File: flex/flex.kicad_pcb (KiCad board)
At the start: 2 copper layers, 68.2 x 125 mm, 11 parts, among them SW1 SW_Push, SW2 SW_Push, SW3 SW_Push

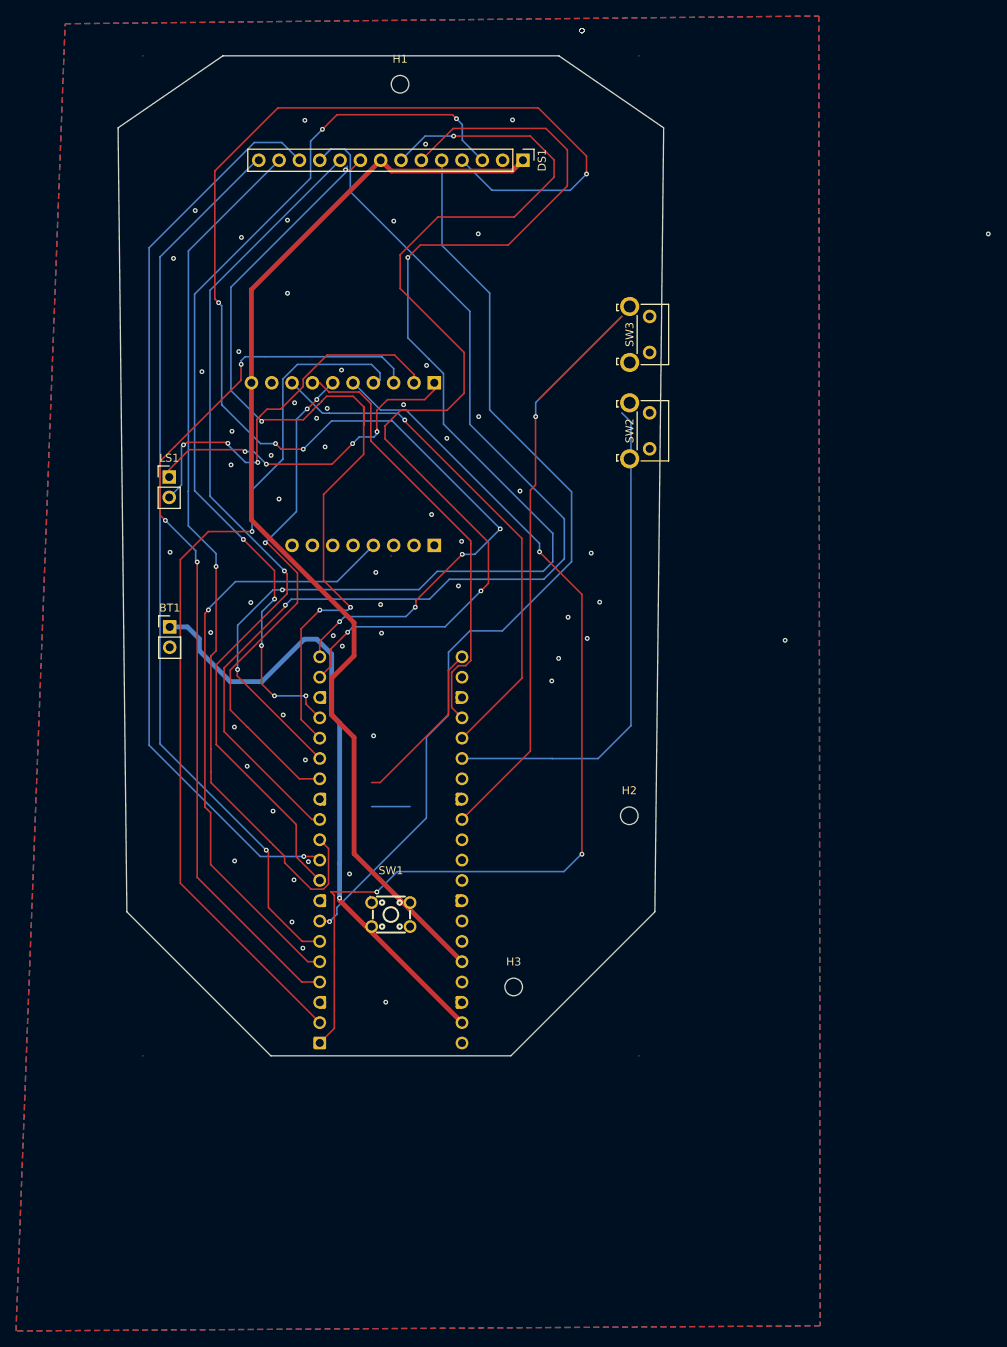
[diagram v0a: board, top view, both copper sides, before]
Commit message: started on firmware
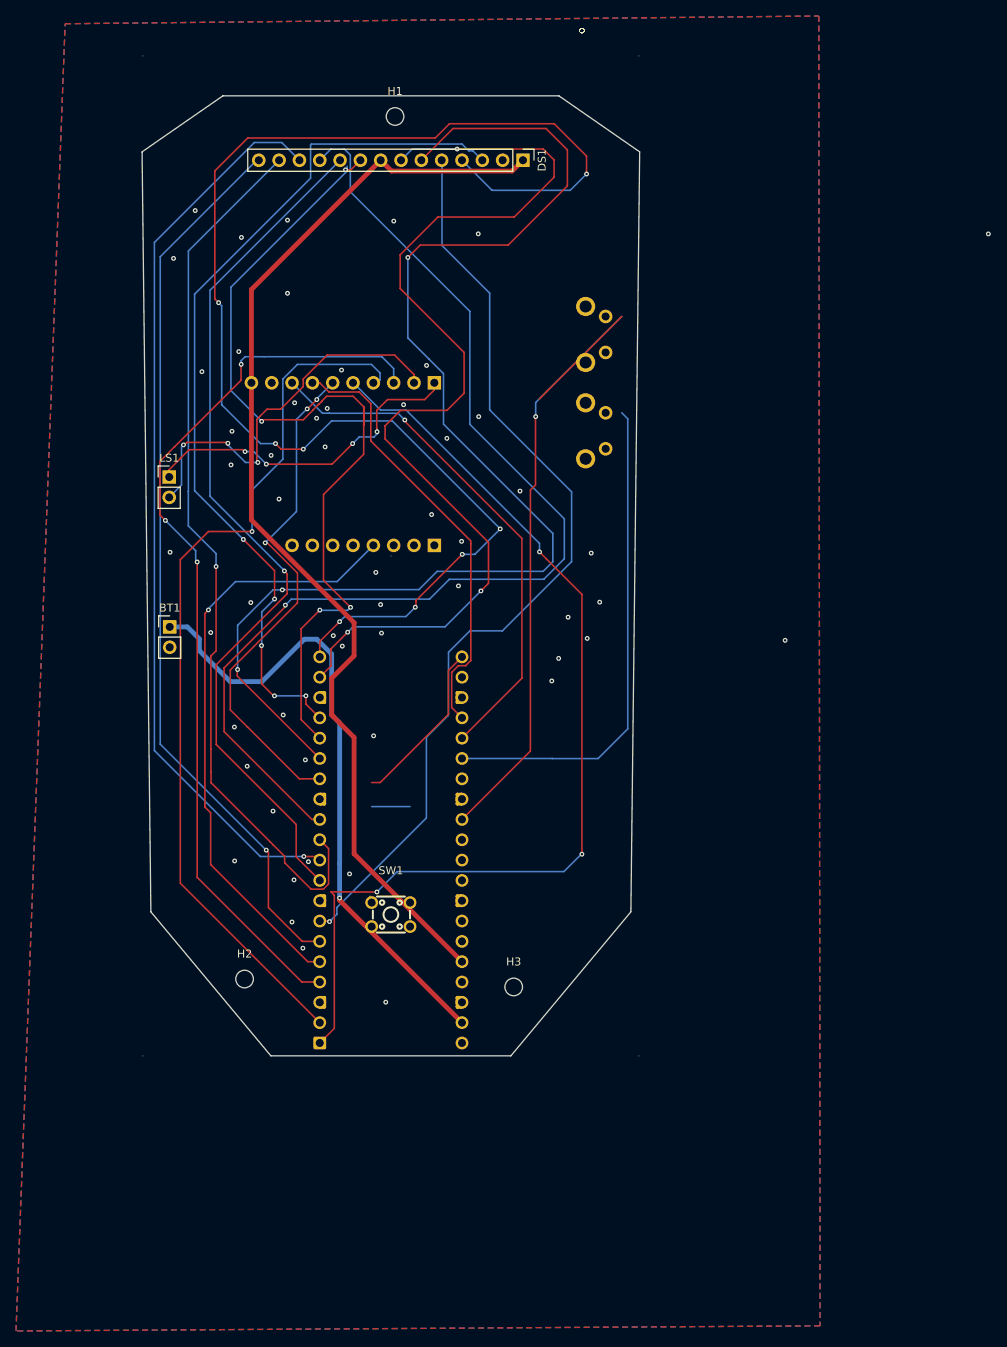
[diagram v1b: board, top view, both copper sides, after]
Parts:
- SW2, SW3: moved to B.Cu
- moved H2 52.2 mm to (84.8, 143.9)
- moved SW3 17.4 mm to (130.0, 77.7), turned to 90 degrees
- moved SW2 9.34 mm to (130.0, 65.6), turned to 90 degrees
- moved H1 4.08 mm to (103.6, 36.1)
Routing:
- net /DISP_CS: track 114.8 -> 110.3 mm, vias 7 -> 5
- net /DISP_RESET: track 177.1 -> 175.5 mm
- net /DISP_SCK: track 131.5 -> 130.1 mm
- net /DISP_T_MOSI: track 114.6 -> 114.1 mm
- net GND: vias 56 -> 53
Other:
- board size 68.2 x 125 mm -> 62.2 x 125 mm

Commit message: added firmware and art
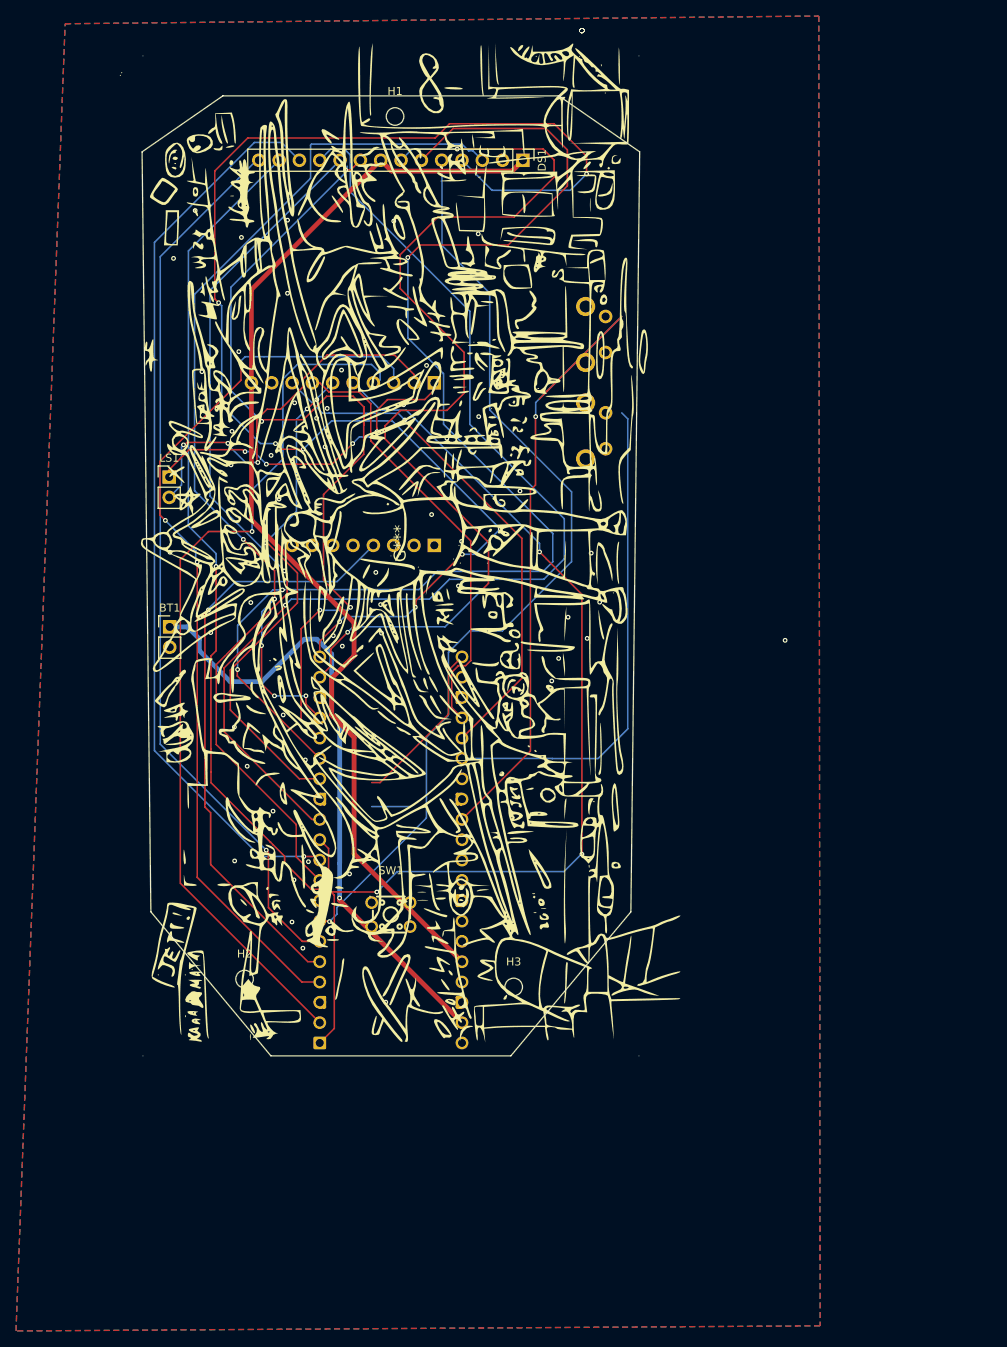
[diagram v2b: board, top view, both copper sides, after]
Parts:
- added G***: LOGO, LOGO, F.Cu at (104.3, 89.5)
- added G***: LOGO, LOGO, B.Cu at (103.9, 89.5)
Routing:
- net (no net): vias 15 -> 14
